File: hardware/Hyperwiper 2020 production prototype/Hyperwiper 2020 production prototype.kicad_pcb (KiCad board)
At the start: 2 copper layers, 87.6 x 59.1 mm, 12 parts, among them K1 Main Power relay, K2 Wiper control relay, Q1 PN2222A, U1 Teensy4.0, U2 Audio board, U3 L7805

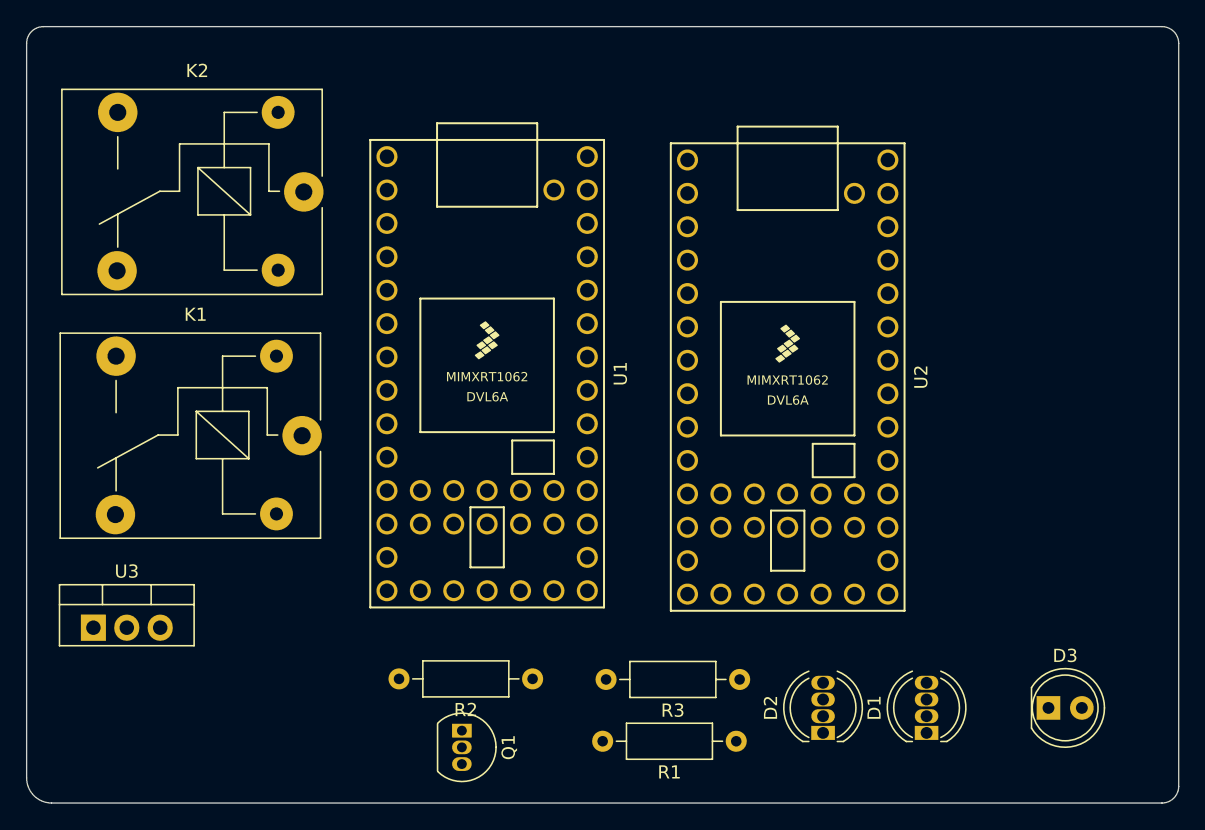
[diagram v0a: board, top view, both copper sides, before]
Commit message: Updates schematic and PCB boards
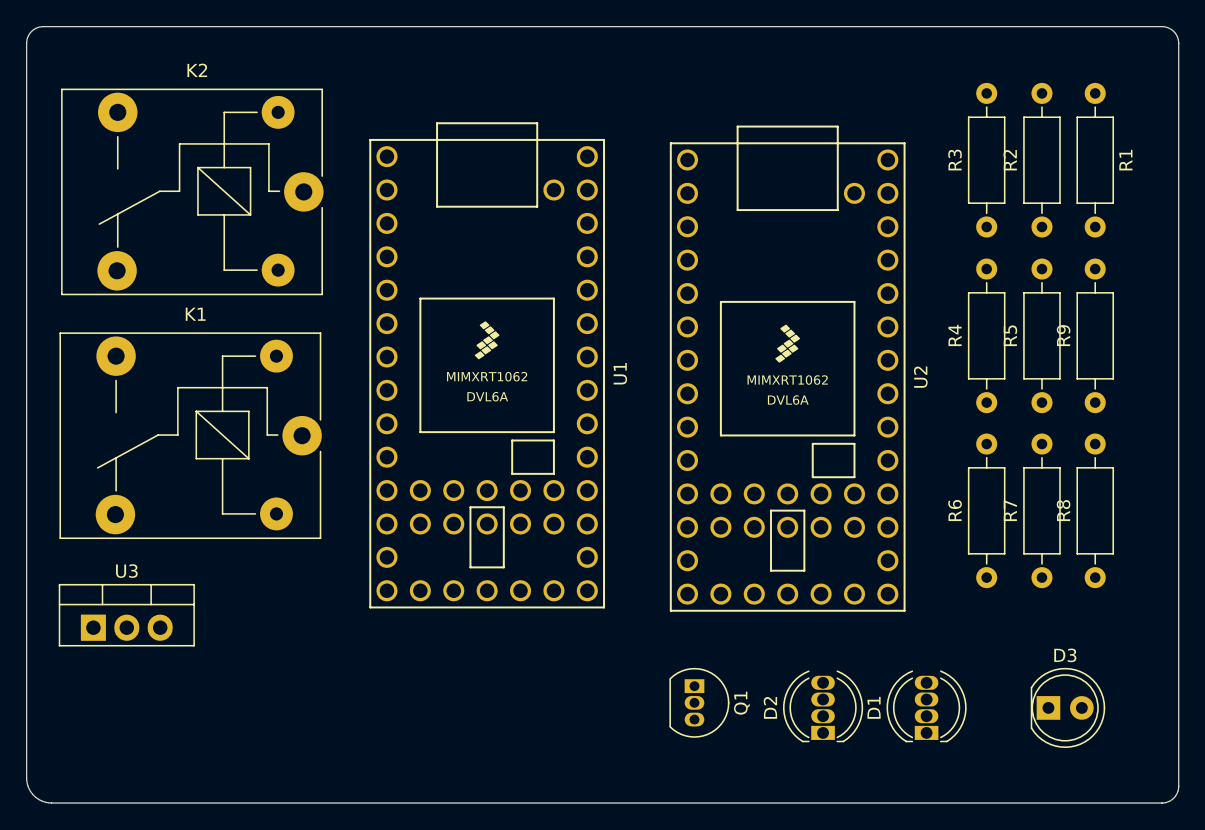
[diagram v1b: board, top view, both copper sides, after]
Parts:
- added R4: R, Resistor_THT:R_Axial_DIN0207_L6.3mm_D2.5mm_P10.16mm_Horizontal, F.Cu at (972.2, 35.0)
- added R5: R, Resistor_THT:R_Axial_DIN0207_L6.3mm_D2.5mm_P10.16mm_Horizontal, F.Cu at (976.4, 35.0)
- added R6: R, Resistor_THT:R_Axial_DIN0207_L6.3mm_D2.5mm_P10.16mm_Horizontal, F.Cu at (972.2, 48.3)
- added R7: R, Resistor_THT:R_Axial_DIN0207_L6.3mm_D2.5mm_P10.16mm_Horizontal, F.Cu at (976.4, 48.3)
- added R8: R, Resistor_THT:R_Axial_DIN0207_L6.3mm_D2.5mm_P10.16mm_Horizontal, F.Cu at (980.4, 48.3)
- added R9: R, Resistor_THT:R_Axial_DIN0207_L6.3mm_D2.5mm_P10.16mm_Horizontal, F.Cu at (980.4, 35.0)
- moved R1 56.3 mm to (980.4, 11.4), turned to -90 degrees
- moved R2 51.8 mm to (976.4, 21.6), turned to 90 degrees
- moved R3 39.2 mm to (972.2, 21.6), turned to 90 degrees
- moved Q1 18.0 mm to (950.0, 56.5)
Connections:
- D1 pad 1: (no net) -> GND
- D1 pad 2: (no net) -> Net-(D1-Pad2)
- D1 pad 3: (no net) -> Net-(D1-Pad3)
- D1 pad 4: (no net) -> Net-(D1-Pad4)
- D2 pad 1: (no net) -> GND
- D2 pad 2: (no net) -> Net-(D2-Pad2)
- D2 pad 3: (no net) -> Net-(D2-Pad3)
- D2 pad 4: (no net) -> Net-(D2-Pad4)
- D3 pad 1: Net-(D3-Pad1) -> GND
- D3 pad 2: GND -> Net-(D3-Pad2)
- K1 pad 1: (no net) -> Net-(K1-Pad1)
- K2 pad 1: (no net) -> Net-(K1-Pad4)
- K2 pad 3: (no net) -> Net-(K1-Pad1)
- R3 pad 1: Net-(D3-Pad1) -> Net-(D3-Pad2)

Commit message: Update Schematics and PCB
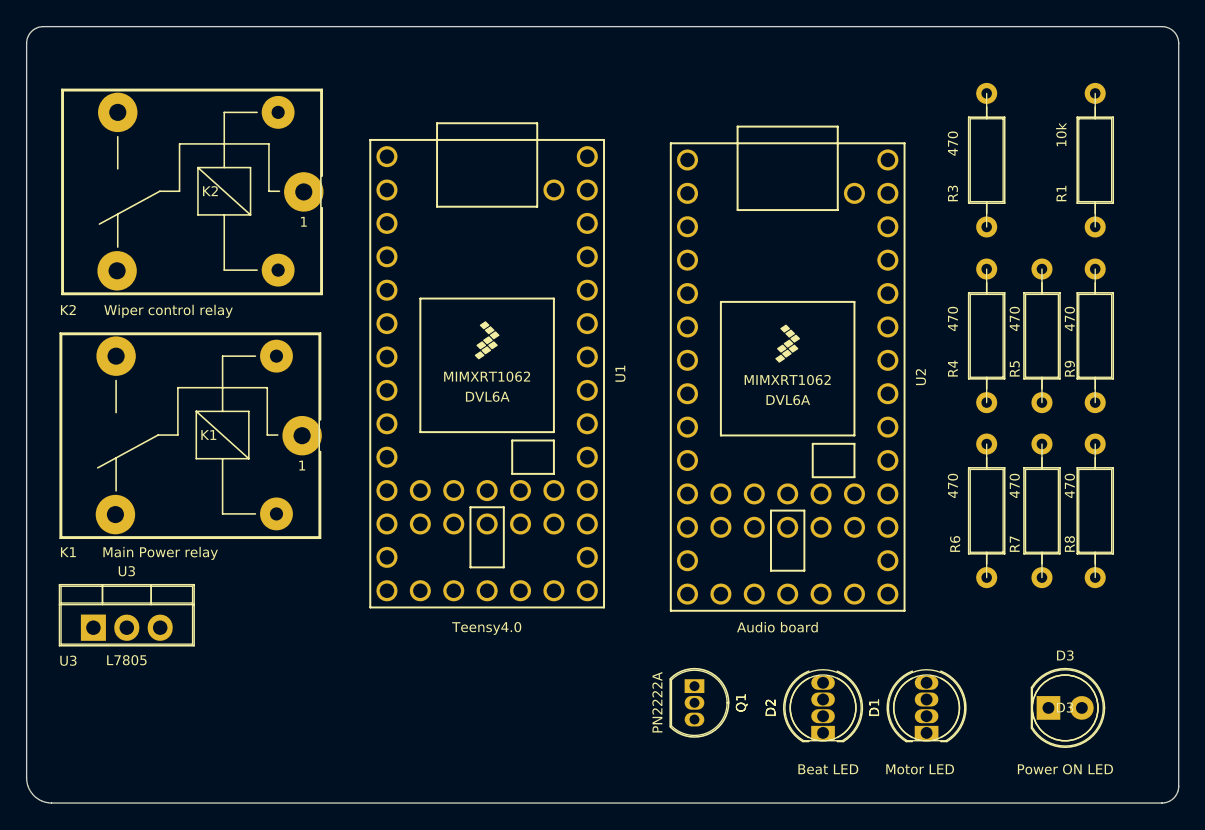
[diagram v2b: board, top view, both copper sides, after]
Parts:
- removed R2: R, Resistor_THT:R_Axial_DIN0207_L6.3mm_D2.5mm_P10.16mm_Horizontal
- R1: value R -> 10k
- R3, R4, R5, R6, R7, R8, R9: value R -> 470
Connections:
- R3 pad 2: Net-(K1-Pad3) -> /33
